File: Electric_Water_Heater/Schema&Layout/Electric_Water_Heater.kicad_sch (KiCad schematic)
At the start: 14 parts, among them J1 Barrel_Jack_Switch, SW1 SW_Push, U1 ATmega32A-P, U2 L7805, Y1 16MHz

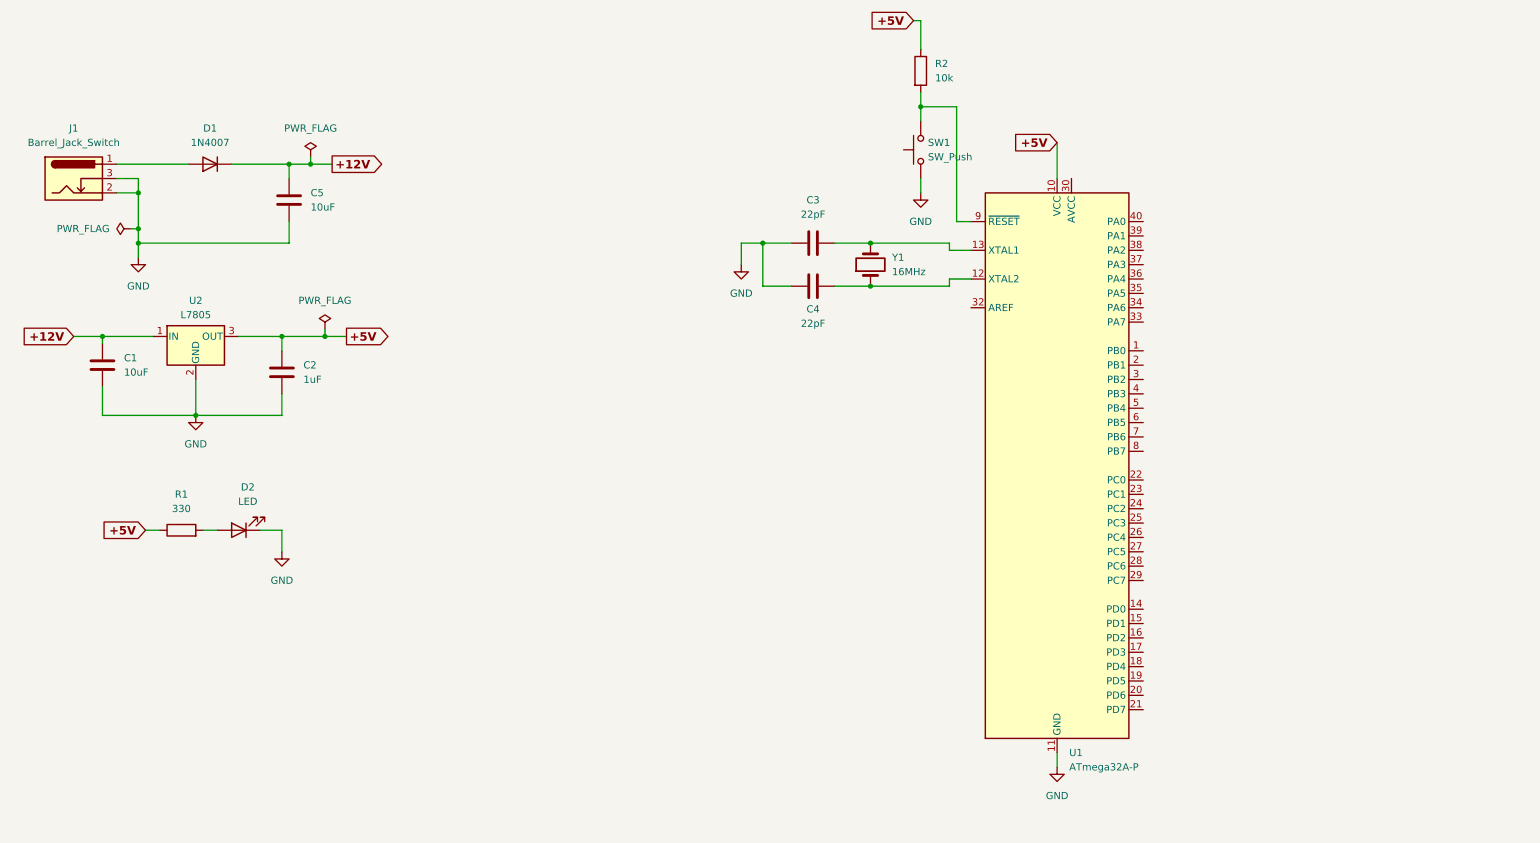
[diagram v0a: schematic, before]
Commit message: New_Update
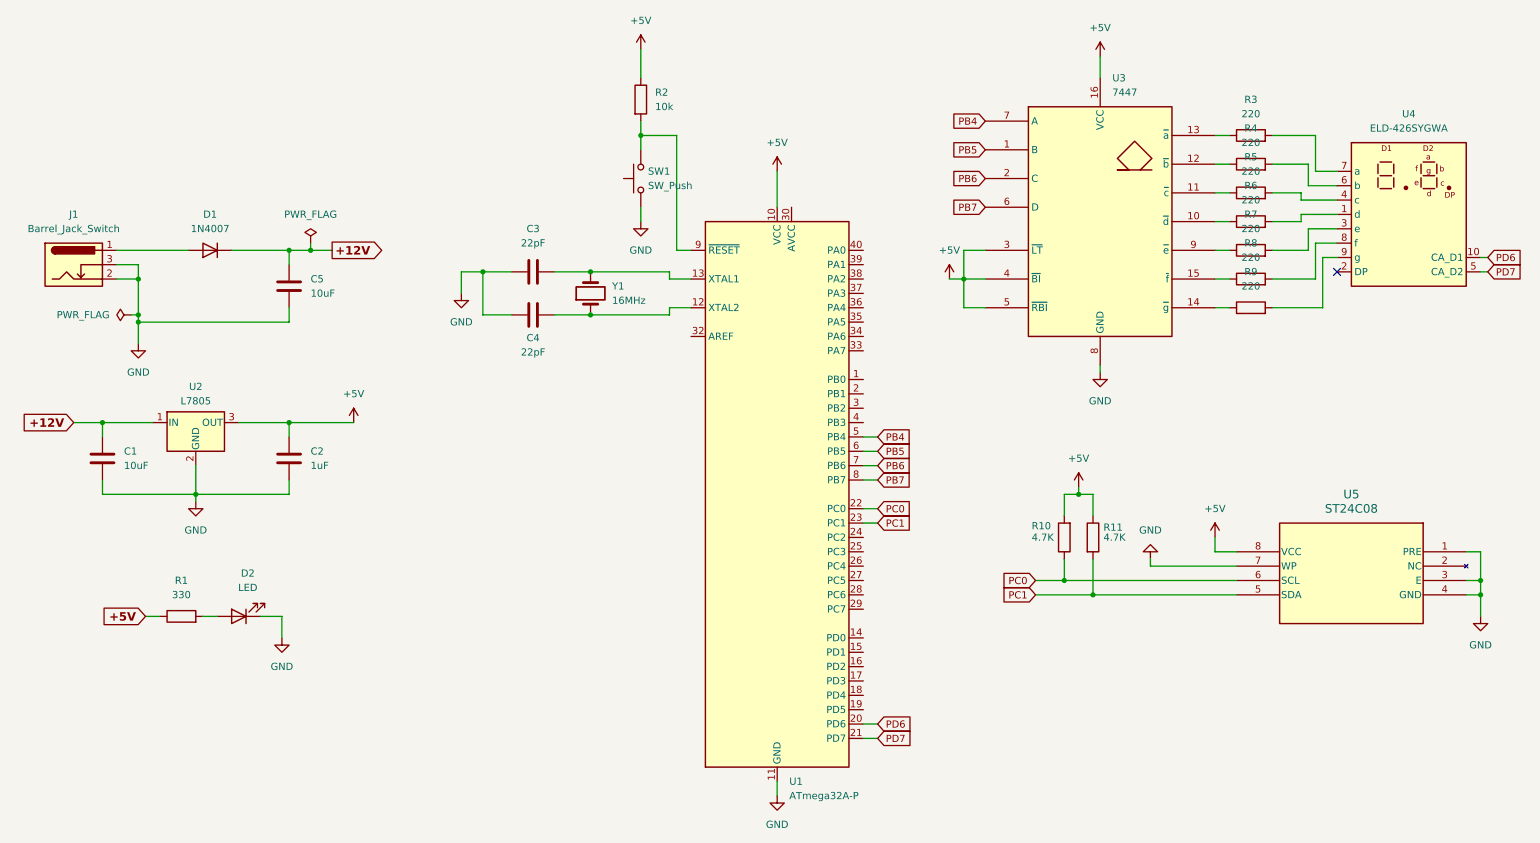
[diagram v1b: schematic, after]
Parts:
- added R10, R11: 4.7K, symbol Device:R
- added R3, R4, R5, R6, R7, R8, R9: 220, symbol Device:R
- added U3: 7447, Decoder:7447, symbol 74xx_IEEE:7447
- added U4: ELD-426SYGWA, Display_7Segment:ELD_426XXXX, symbol Display_Character:ELD-426SYGWA
- added U5: ST24C08, Memory:ST24C08, symbol Memory_EEPROM:ST24C08
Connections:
- net +5V: now also R10.2, R11.1, U3.16 (VCC), U3.3 (~{LT}), U3.4 (~{BI}), U3.5 (~{RBI}), U5.8 (VCC)
- net GND: now also U3.8 (GND), U5.1 (PRE), U5.3 (E), U5.4 (GND), U5.7 (WP)
- net PD6: now reaches U1.20 (PD6)
- net PD6: now also U4.10 (CA_D1)
- net PD7: now reaches U1.21 (PD7)
- net PD7: now also U4.5 (CA_D2)
- net PC0: now reaches U1.22 (PC0)
- net PC0: now also R10.1, U5.6 (SCL)
- net PC1: now reaches U1.23 (PC1)
- net PC1: now also R11.2, U5.5 (SDA)
- net PB4: now reaches U1.5 (PB4)
- net PB4: now also U3.7 (A)
- net PB5: now reaches U1.6 (PB5)
- net PB5: now also U3.1 (B)
- net PB6: now reaches U1.7 (PB6)
- net PB6: now also U3.2 (C)
- net PB7: now reaches U1.8 (PB7)
- net PB7: now also U3.6 (D)
- new net: R8.1, U3.15 (~{f})
- new net: R8.2, U4.8 (f)
- new net: R6.1, U3.10 (~{d})
- new net: R5.1, U3.11 (~{c})
- new net: R4.1, U3.12 (~{b})
- new net: R3.1, U3.13 (~{a})
- new net: R9.1, U3.14 (~{g})
- new net: R7.1, U3.9 (~{e})
- new net: R5.2, U4.4 (c)
- new net: R6.2, U4.1 (d)
- new net: R7.2, U4.3 (e)
- new net: R4.2, U4.6 (b)
- new net: R3.2, U4.7 (a)
- new net: R9.2, U4.9 (g)
- no-connect marks 0 -> 1
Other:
- moved on the sheet: C1, C2, C3, C4, C5, D1, D2, J1, R1, R2, SW1, U1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
